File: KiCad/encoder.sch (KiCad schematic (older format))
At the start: 24 parts, among them P11 CONN_01X08, P12 ISP, P13 FTDI, P14 ENC_SS, SW1 ENC_RST, U5 ATMEGA328P, U6 3V3, X2 8MHz

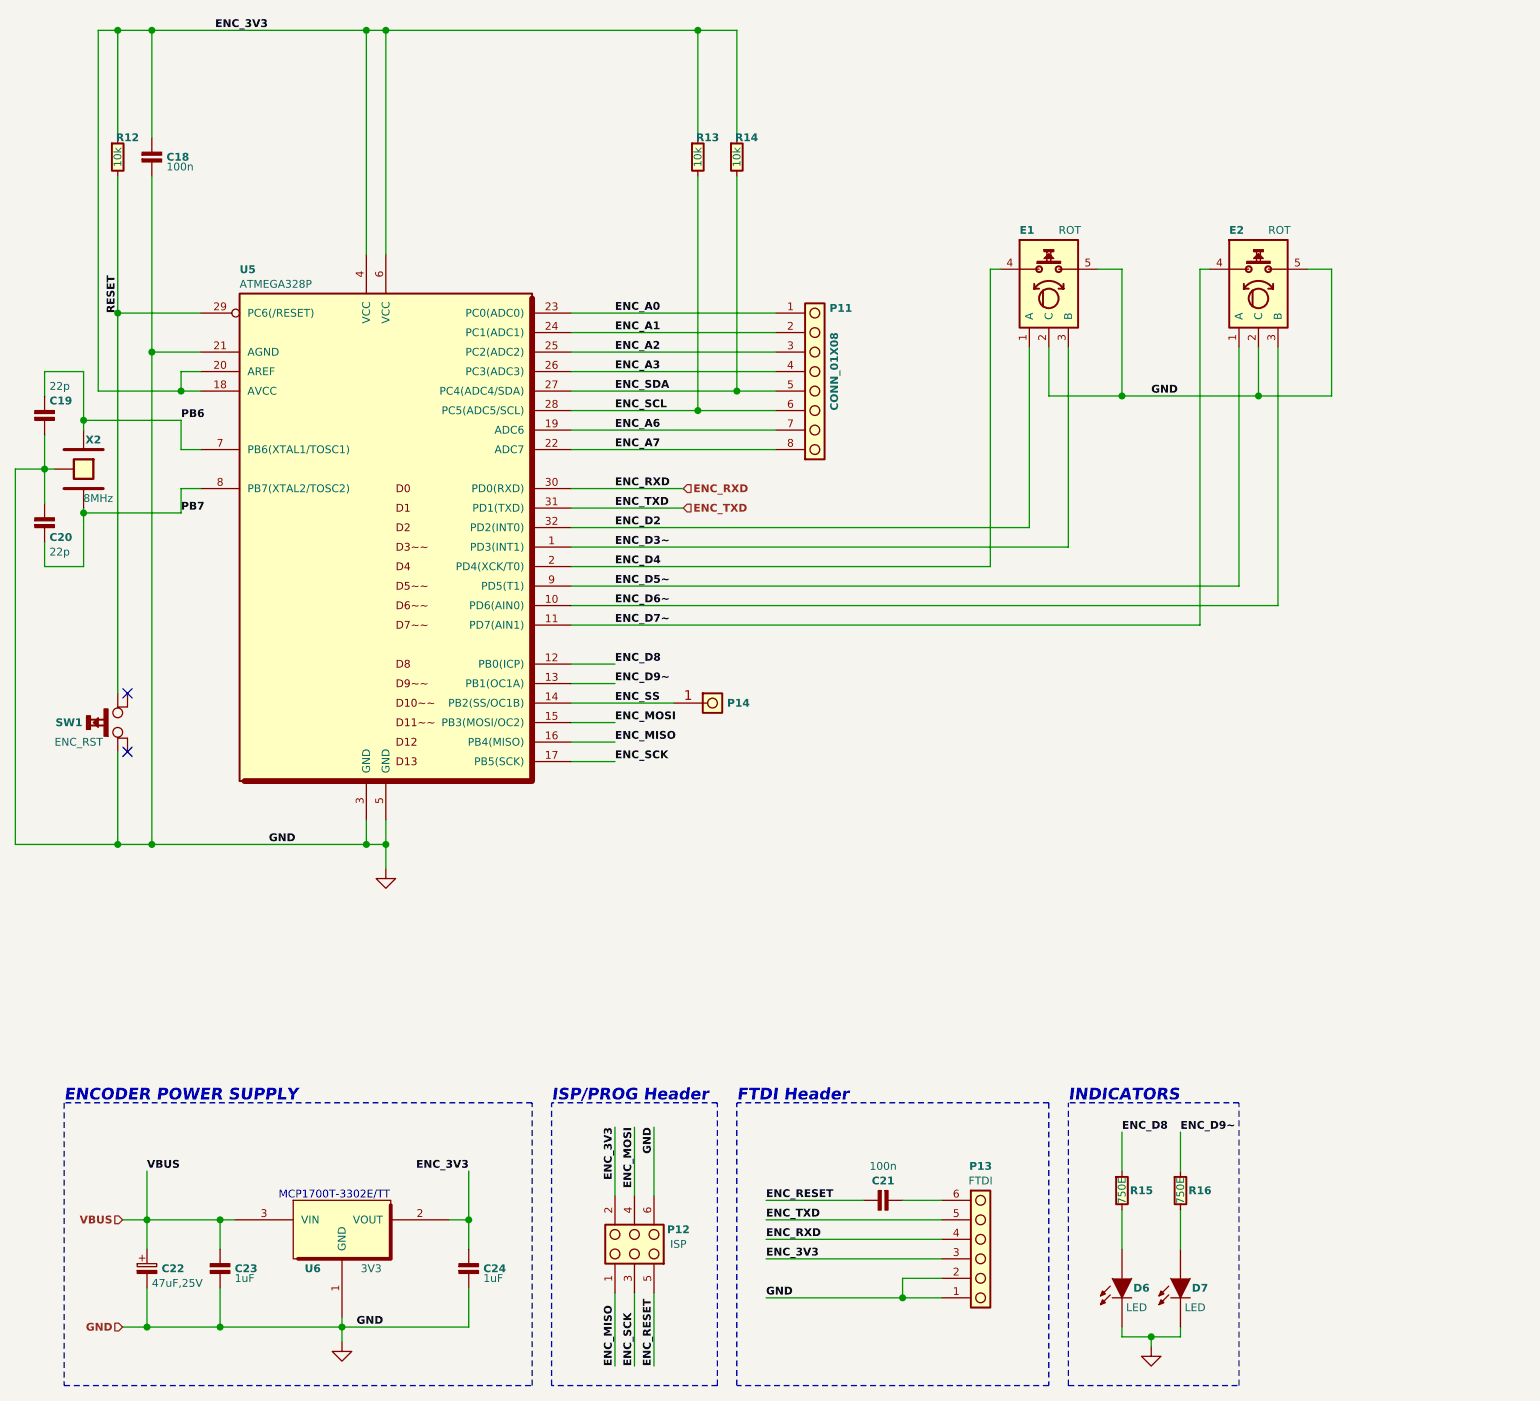
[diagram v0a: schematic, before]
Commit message: schematic, work in progress
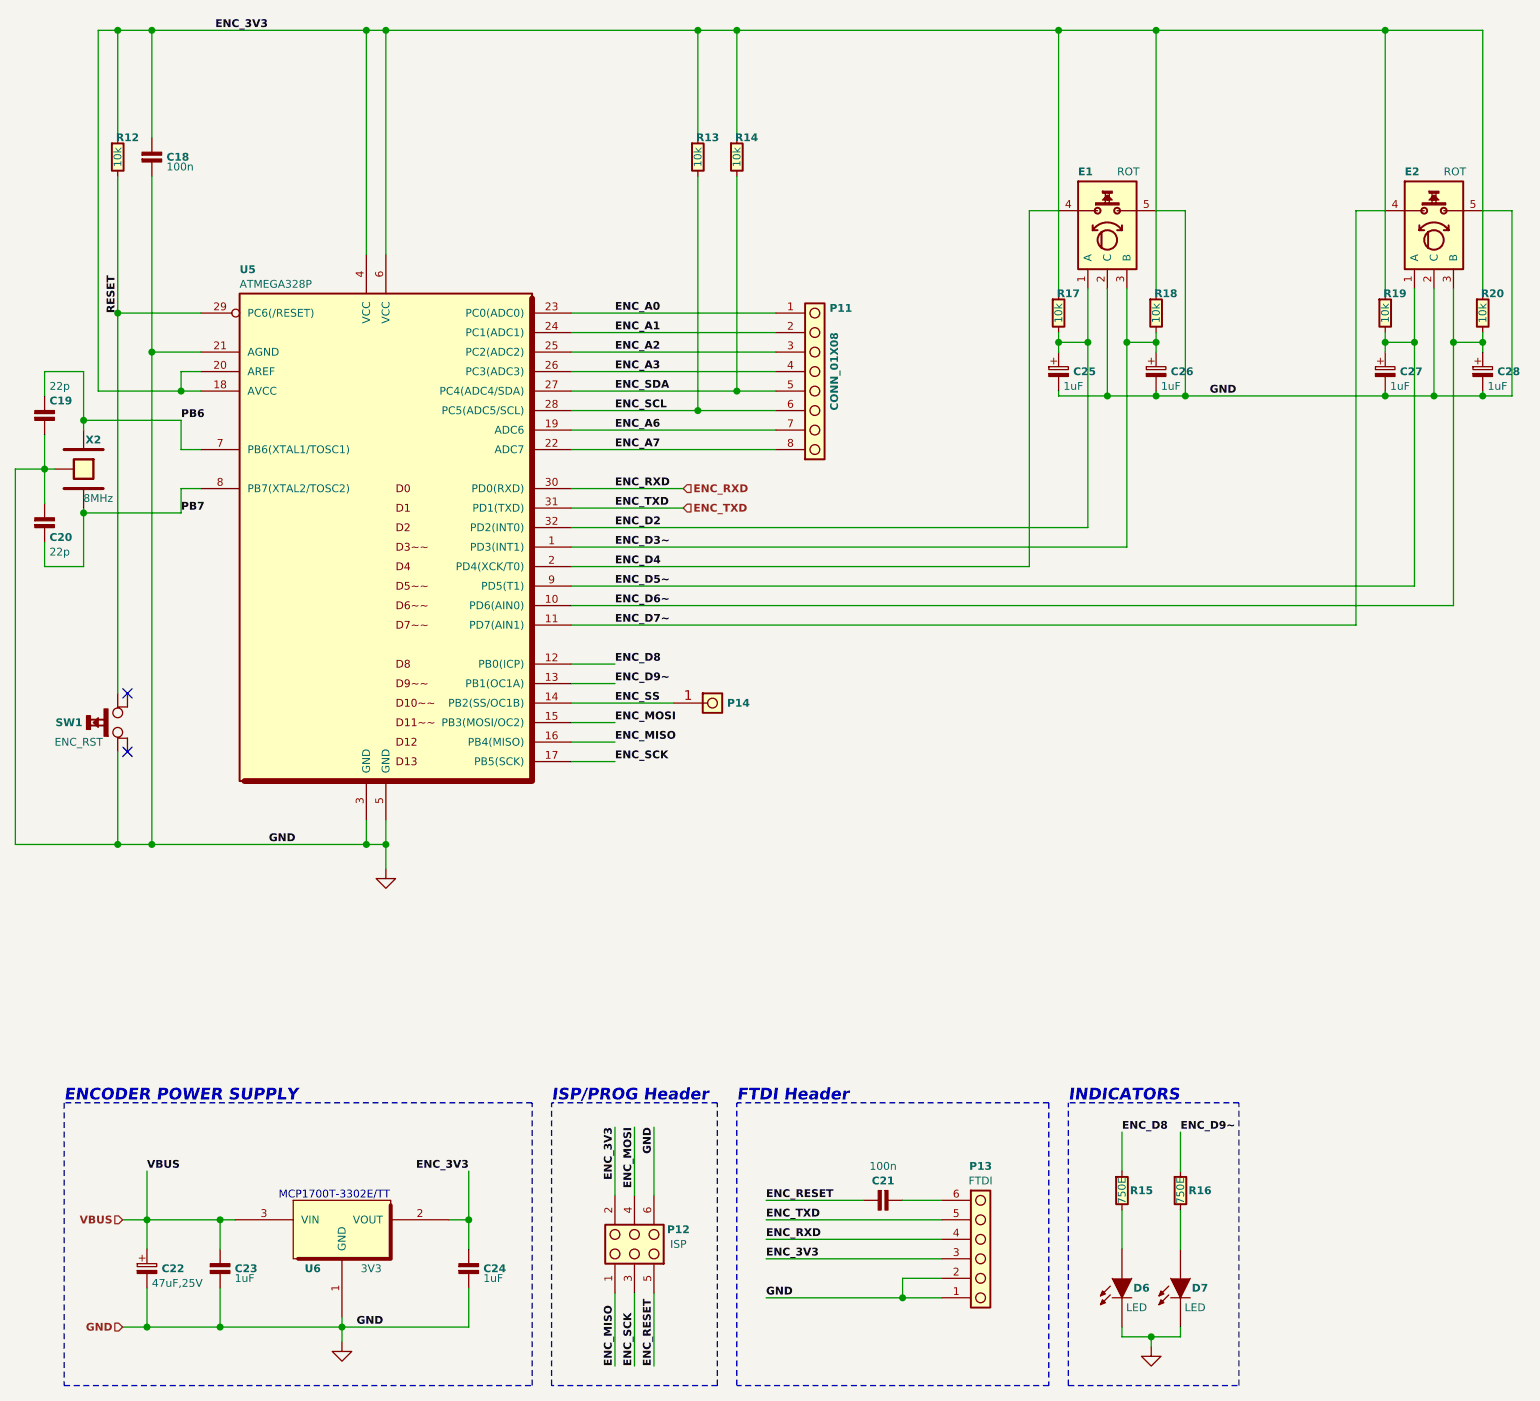
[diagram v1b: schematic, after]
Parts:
- added C25, C26, C27, C28: 1uF, ArthurC Lib:C_ELCO_SMD, symbol CP_Small
- added R17, R18, R19, R20: 10k, ArthurC Lib:r_0805, symbol R_Small
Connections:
- net ENC_3V3: now also R17.1, R18.1, R19.1, R20.1
- net ENC_D2: now also C25.1, R17.2
- net ENC_D3~~: now also C26.1, R18.2
- net ENC_D5~~: now also C27.1, R19.2
- net ENC_D6~~: now also C28.1, R20.2
- net GND: now also C25.2, C26.2, C27.2, C28.2
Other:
- moved on the sheet: E1, E2
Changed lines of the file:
@@
 LIBS:velokey
 LIBS:power
-LIBS:PiPower_sch
-LIBS:arthurc
 LIBS:velokey-cache
 EELAYER 25 0
@@
 Connection ~ 1600 6900
 Wire Wire Line
-	3400 3350 5750 3350
-Wire Wire Line
-	3400 3550 5550 3550
+	6050 3350 3400 3350
+Wire Wire Line
+	3400 3550 5750 3550
 Connection ~ 1075 800
 Wire Wire Line
@@
 	4250 800  4250 1350
 Wire Wire Line
-	3400 3450 5950 3450
+	6250 3450 3400 3450
 Wire Wire Line
 	3400 3250 3975 3250
@@
 	3400 4050 3625 4050
 Wire Wire Line
-	3400 3850 6625 3850
-Wire Wire Line
-	3400 3750 7025 3750
-Wire Wire Line
-	3400 3650 6825 3650
+	3400 3850 7425 3850
+Wire Wire Line
+	7925 3750 3400 3750
+Wire Wire Line
+	7725 3650 3400 3650
 Wire Wire Line
 	3400 2850 4450 2850
@@
 	2775 6900 2875 6900
 Wire Wire Line
-	975  800  4250 800
+	975  800  8075 800
 Wire Wire Line
 	4400 7300 5300 7300
@@
 L ROT E1
 U 1 1 56A8236D
-P 5850 2175
-F 0 "E1" H 5700 2525 40  0000 L CNB
-F 1 "ROT" H 5900 2525 40  0000 L CNN
-F 2 "" H 5850 2175 40  0000 C CNN
-F 3 "" H 5850 2175 40  0000 C CNN
-F 4 "mfr_pn" H 5850 2175 40  0001 C CNN "manf#"
-	1    5850 2175
+P 6150 1875
+F 0 "E1" H 6000 2225 40  0000 L CNB
+F 1 "ROT" H 6200 2225 40  0000 L CNN
+F 2 "" H 6150 1875 40  0000 C CNN
+F 3 "" H 6150 1875 40  0000 C CNN
+F 4 "mfr_pn" H 6150 1875 40  0001 C CNN "manf#"
+	1    6150 1875
 	1    0    0    -1
 $EndComp
@@
 L ROT E2
 U 1 1 56A824EE
-P 6925 2175
-F 0 "E2" H 6775 2525 40  0000 L CNB
-F 1 "ROT" H 6975 2525 40  0000 L CNN
-F 2 "" H 6925 2175 40  0000 C CNN
-F 3 "" H 6925 2175 40  0000 C CNN
-F 4 "mfr_pn" H 6925 2175 40  0001 C CNN "manf#"
-	1    6925 2175
-	1    0    0    -1
-$EndComp
-Wire Wire Line
-	6100 2025 6225 2025
-Wire Wire Line
-	6225 2025 6225 2675
-Wire Wire Line
-	5850 2675 7300 2675
-Wire Wire Line
-	5850 2675 5850 2425
-Wire Wire Line
-	7175 2025 7300 2025
-Wire Wire Line
-	7300 2025 7300 2675
-Wire Wire Line
-	6925 2675 6925 2425
-Connection ~ 6225 2675
-Connection ~ 6925 2675
-Wire Wire Line
-	5750 3350 5750 2425
-Wire Wire Line
-	5950 3450 5950 2425
-Wire Wire Line
-	5550 3550 5550 2025
-Wire Wire Line
-	5550 2025 5600 2025
-Wire Wire Line
-	6825 3650 6825 2425
-Wire Wire Line
-	7025 3750 7025 2425
-Wire Wire Line
-	6675 2025 6625 2025
-Wire Wire Line
-	6625 2025 6625 3850
-Text Label 6375 2675 0    40   ~ 8
+P 7825 1875
+F 0 "E2" H 7675 2225 40  0000 L CNB
+F 1 "ROT" H 7875 2225 40  0000 L CNN
+F 2 "" H 7825 1875 40  0000 C CNN
+F 3 "" H 7825 1875 40  0000 C CNN
+F 4 "mfr_pn" H 7825 1875 40  0001 C CNN "manf#"
+	1    7825 1875
+	1    0    0    -1
+$EndComp
+Wire Wire Line
+	6400 1725 6550 1725
+Wire Wire Line
+	6550 1725 6550 2675
+Wire Wire Line
+	5900 2675 8225 2675
+Wire Wire Line
+	6150 2675 6150 2125
+Wire Wire Line
+	8075 1725 8225 1725
+Wire Wire Line
+	8225 1725 8225 2675
+Wire Wire Line
+	7825 2675 7825 2125
+Connection ~ 6550 2675
+Connection ~ 7825 2675
+Wire Wire Line
+	6050 2125 6050 3350
+Wire Wire Line
+	6250 2125 6250 3450
+Wire Wire Line
+	5750 3550 5750 1725
+Wire Wire Line
+	5750 1725 5900 1725
+Wire Wire Line
+	7725 2125 7725 3650
+Wire Wire Line
+	7925 2125 7925 3750
+Wire Wire Line
+	7575 1725 7425 1725
+Wire Wire Line
+	7425 1725 7425 3850
+Text Label 6675 2675 0    40   ~ 8
 GND
 Text Label 3625 3550 0    40   ~ 8
@@
 	1    0    0    -1
 $EndComp
+$Comp
+L CP_Small C25
+U 1 1 56A75B87
+P 5900 2550
+F 0 "C25" H 5975 2550 40  0000 L CNB
+F 1 "1uF" H 5925 2475 40  0000 L CNN
+F 2 "ArthurC Lib:C_ELCO_SMD" H 5900 2550 60  0001 C CNN
+F 3 "" H 5900 2550 60  0000 C CNN
+F 4 "mfr_pn" H 5900 2550 60  0001 C CNN "manf#"
+	1    5900 2550
+	1    0    0    -1
+$EndComp
+$Comp
+L CP_Small C26
+U 1 1 56A7615B
+P 6400 2550
+F 0 "C26" H 6475 2550 40  0000 L CNB
+F 1 "1uF" H 6425 2475 40  0000 L CNN
+F 2 "ArthurC Lib:C_ELCO_SMD" H 6400 2550 60  0001 C CNN
+F 3 "" H 6400 2550 60  0000 C CNN
+F 4 "mfr_pn" H 6400 2550 60  0001 C CNN "manf#"
+	1    6400 2550
+	1    0    0    -1
+$EndComp
+$Comp
+L CP_Small C27
+U 1 1 56A7636B
+P 7575 2550
+F 0 "C27" H 7650 2550 40  0000 L CNB
+F 1 "1uF" H 7600 2475 40  0000 L CNN
+F 2 "ArthurC Lib:C_ELCO_SMD" H 7575 2550 60  0001 C CNN
+F 3 "" H 7575 2550 60  0000 C CNN
+F 4 "mfr_pn" H 7575 2550 60  0001 C CNN "manf#"
+	1    7575 2550
+	1    0    0    -1
+$EndComp
+$Comp
+L CP_Small C28
+U 1 1 56A76452
+P 8075 2550
+F 0 "C28" H 8150 2550 40  0000 L CNB
+F 1 "1uF" H 8100 2475 40  0000 L CNN
+F 2 "ArthurC Lib:C_ELCO_SMD" H 8075 2550 60  0001 C CNN
+F 3 "" H 8075 2550 60  0000 C CNN
+F 4 "mfr_pn" H 8075 2550 60  0001 C CNN "manf#"
+	1    8075 2550
+	1    0    0    -1
+$EndComp
+Wire Wire Line
+	7575 2350 7575 2450
+Wire Wire Line
+	7575 2400 7725 2400
+Connection ~ 7725 2400
+Wire Wire Line
+	7925 2400 8075 2400
+Wire Wire Line
+	8075 2350 8075 2450
+Connection ~ 7925 2400
+Wire Wire Line
+	8075 2650 8075 2675
+Connection ~ 8075 2675
+Wire Wire Line
+	7575 2650 7575 2675
+Connection ~ 7575 2675
+Wire Wire Line
+	6400 2350 6400 2450
+Wire Wire Line
+	6400 2400 6250 2400
+Connection ~ 6250 2400
+Wire Wire Line
+	5900 2350 5900 2450
+Wire Wire Line
+	5900 2400 6050 2400
+Connection ~ 6050 2400
+Wire Wire Line
+	5900 2650 5900 2675
+Connection ~ 6150 2675
+Wire Wire Line
+	6400 2650 6400 2675
+Connection ~ 6400 2675
+$Comp
+L R_Small R17
+U 1 1 56A76C80
+P 5900 2250
+F 0 "R17" H 5950 2350 40  0000 C CNB
+F 1 "10k" V 5900 2250 40  0000 C CNN
+F 2 "ArthurC Lib:r_0805" H 5900 2250 60  0001 C CNN
+F 3 "" H 5900 2250 60  0001 C CNN
+F 4 "mfr_pn" H 5900 2250 60  0001 C CNN "manf#"
+	1    5900 2250
+	1    0    0    -1
+$EndComp
+$Comp
+L R_Small R18
+U 1 1 56A77454
+P 6400 2250
+F 0 "R18" H 6450 2350 40  0000 C CNB
+F 1 "10k" V 6400 2250 40  0000 C CNN
+F 2 "ArthurC Lib:r_0805" H 6400 2250 60  0001 C CNN
+F 3 "" H 6400 2250 60  0001 C CNN
+F 4 "mfr_pn" H 6400 2250 60  0001 C CNN "manf#"
+	1    6400 2250
+	1    0    0    -1
+$EndComp
+$Comp
+L R_Small R19
+U 1 1 56A774E4
+P 7575 2250
+F 0 "R19" H 7625 2350 40  0000 C CNB
+F 1 "10k" V 7575 2250 40  0000 C CNN
+F 2 "ArthurC Lib:r_0805" H 7575 2250 60  0001 C CNN
+F 3 "" H 7575 2250 60  0001 C CNN
+F 4 "mfr_pn" H 7575 2250 60  0001 C CNN "manf#"
+	1    7575 2250
+	1    0    0    -1
+$EndComp
+$Comp
+L R_Small R20
+U 1 1 56A77700
+P 8075 2250
+F 0 "R20" H 8125 2350 40  0000 C CNB
+F 1 "10k" V 8075 2250 40  0000 C CNN
+F 2 "ArthurC Lib:r_0805" H 8075 2250 60  0001 C CNN
+F 3 "" H 8075 2250 60  0001 C CNN
+F 4 "mfr_pn" H 8075 2250 60  0001 C CNN "manf#"
+	1    8075 2250
+	1    0    0    -1
+$EndComp
+Connection ~ 8075 2400
+Connection ~ 7575 2400
+Connection ~ 6400 2400
+Connection ~ 5900 2400
+Wire Wire Line
+	8075 800  8075 2150
+Connection ~ 4250 800
+Wire Wire Line
+	7575 2150 7575 800
+Connection ~ 7575 800
+Wire Wire Line
+	6400 2150 6400 800
+Connection ~ 6400 800
+Wire Wire Line
+	5900 2150 5900 800
+Connection ~ 5900 800
 $EndSCHEMATC
